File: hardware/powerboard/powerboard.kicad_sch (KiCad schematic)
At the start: 74 parts, among them J1 USB_B_Micro, J10 5V, J11 3V3, J2 Boot, J3 Power, J4 Display, J5 Debug, J6 SPI_1, J7 UART_0, J8 I2C_0, J9 I2C_1, SW1 Oct_Up, SW2 RESET, SW3 Oct_Down, SW4 RotaryEncoder_Switch, U2 MCP1603, U3 RP2040, U4 W25Q128JVSIM, Y1 Crystal_GND24

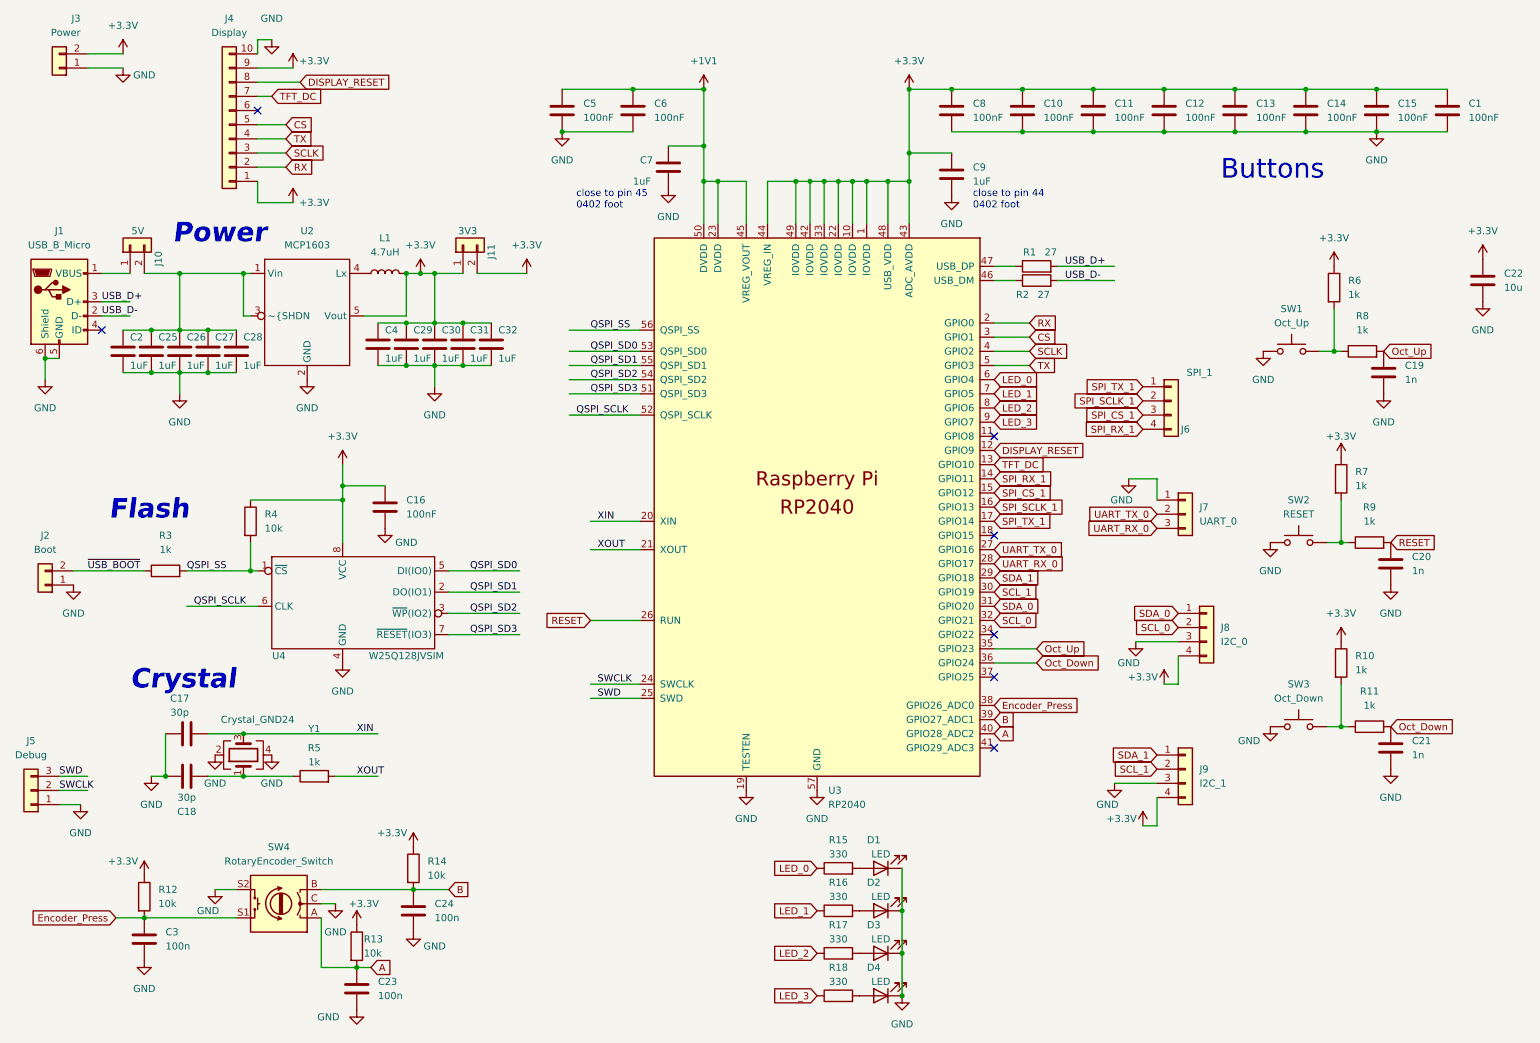
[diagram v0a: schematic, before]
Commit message: Gerbers and pick and place generated
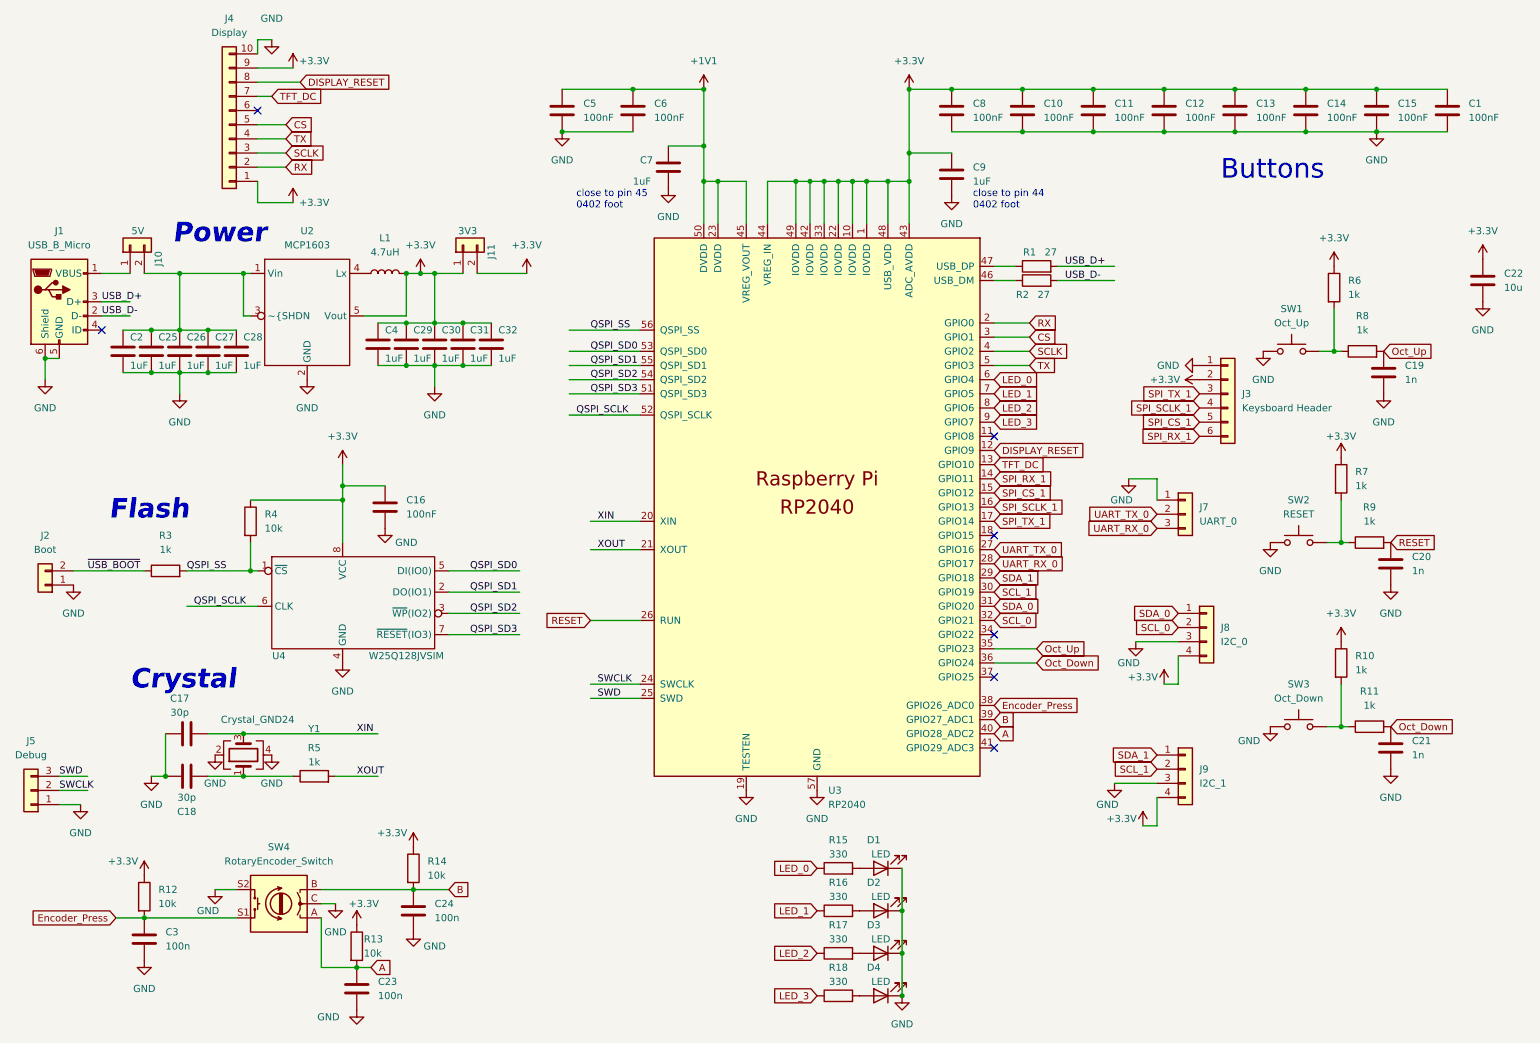
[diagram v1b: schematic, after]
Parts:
- removed J3: Power, Connector_PinHeader_2.54mm:PinHeader_1x02_P2.54mm_Horizontal, symbol Connector_Generic:Conn_01x02
- removed J6: SPI_1, Connector_PinHeader_2.54mm:PinHeader_1x04_P2.54mm_Horizontal, symbol Connector_Generic:Conn_01x04
- added J3: Keysboard Header, Connector_PinHeader_2.54mm:PinHeader_1x06_P2.54mm_Horizontal, symbol Connector_Generic:Conn_01x06
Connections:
- net +3.3V: now also J3.2 (Pin_2)
- net GND: now also J3.1 (Pin_1)
- net SPI_CS_1: now also J3.5 (Pin_5)
- net SPI_RX_1: now also J3.6 (Pin_6)
- net SPI_SCLK_1: now also J3.4 (Pin_4)
- net SPI_TX_1: now also J3.3 (Pin_3)
